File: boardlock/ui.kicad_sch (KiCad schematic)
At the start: 5 parts

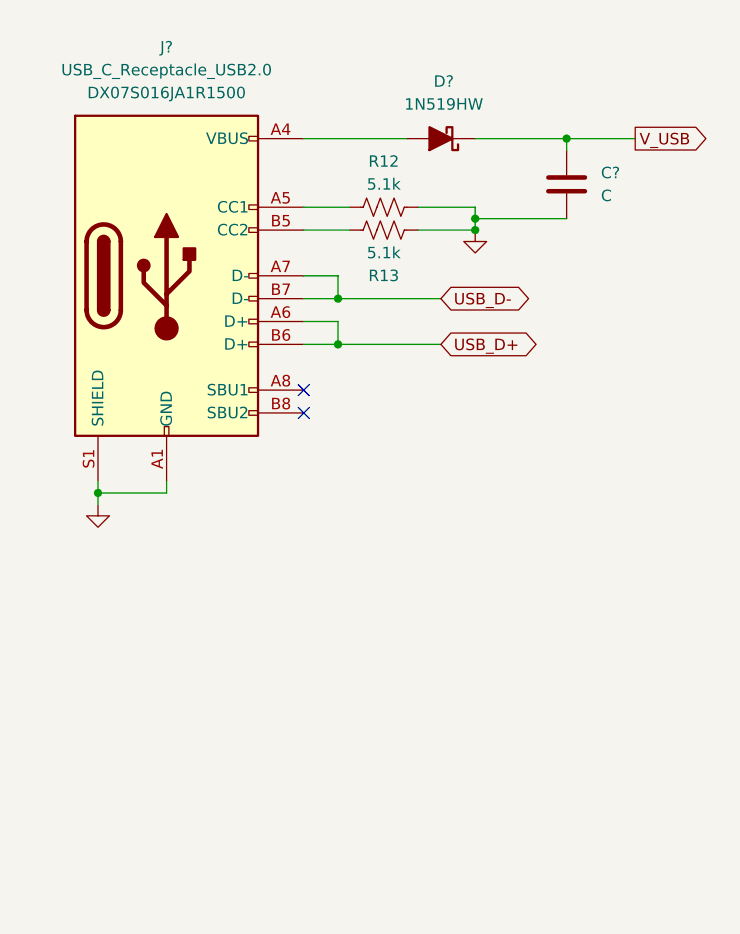
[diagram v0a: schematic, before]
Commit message: more Zecong edits
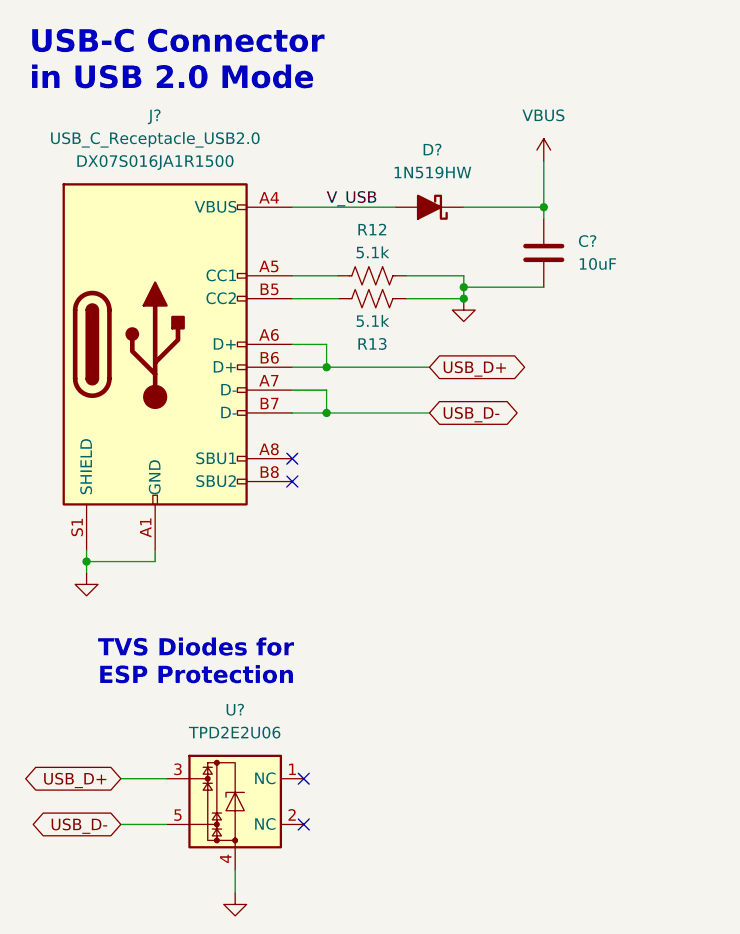
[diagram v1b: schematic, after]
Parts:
- removed C?: C, symbol Device:C
- added C?: 10uF, symbol Device:C
- added U?: TPD2E2U06, Package_TO_SOT_SMD:SOT-543, symbol Power_Protection:TPD2E2U06
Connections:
- net GND: now also C?.2, U?.4
- net USB_D+: now also U?.3
- net USB_D-: now also U?.5
- net V_USB: now also D?.2 (A), J?.A4 (VBUS), J?.A9 (VBUS), J?.B4 (VBUS), J?.B9 (VBUS); no longer D?.1 (K)
- new net VBUS: C?.1, D?.1 (K)
- no-connect marks 2 -> 4
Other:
- note added: "TVS Diodes for ESP Protection"
- note added: "USB-C Connector in USB 2.0 Mode"
- moved on the sheet: D?, J?, R12, R13

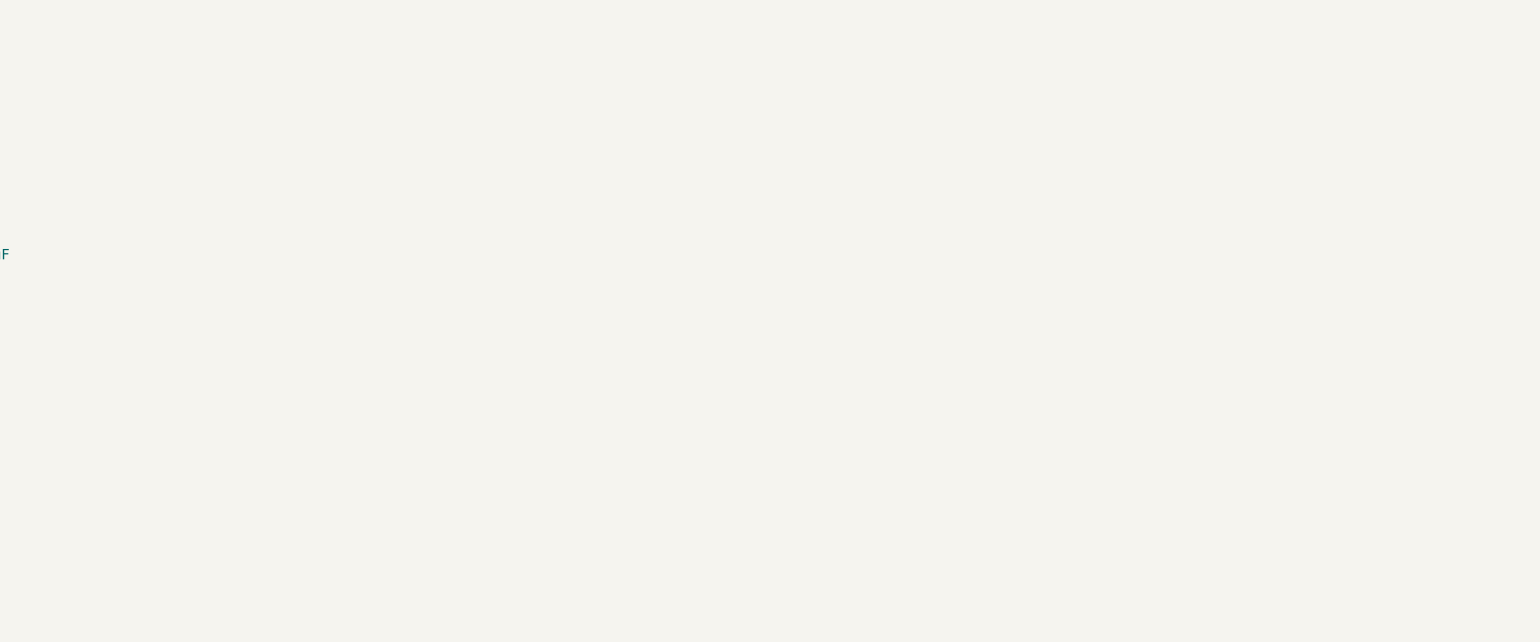
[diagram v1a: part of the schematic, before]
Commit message: buttons and stuff
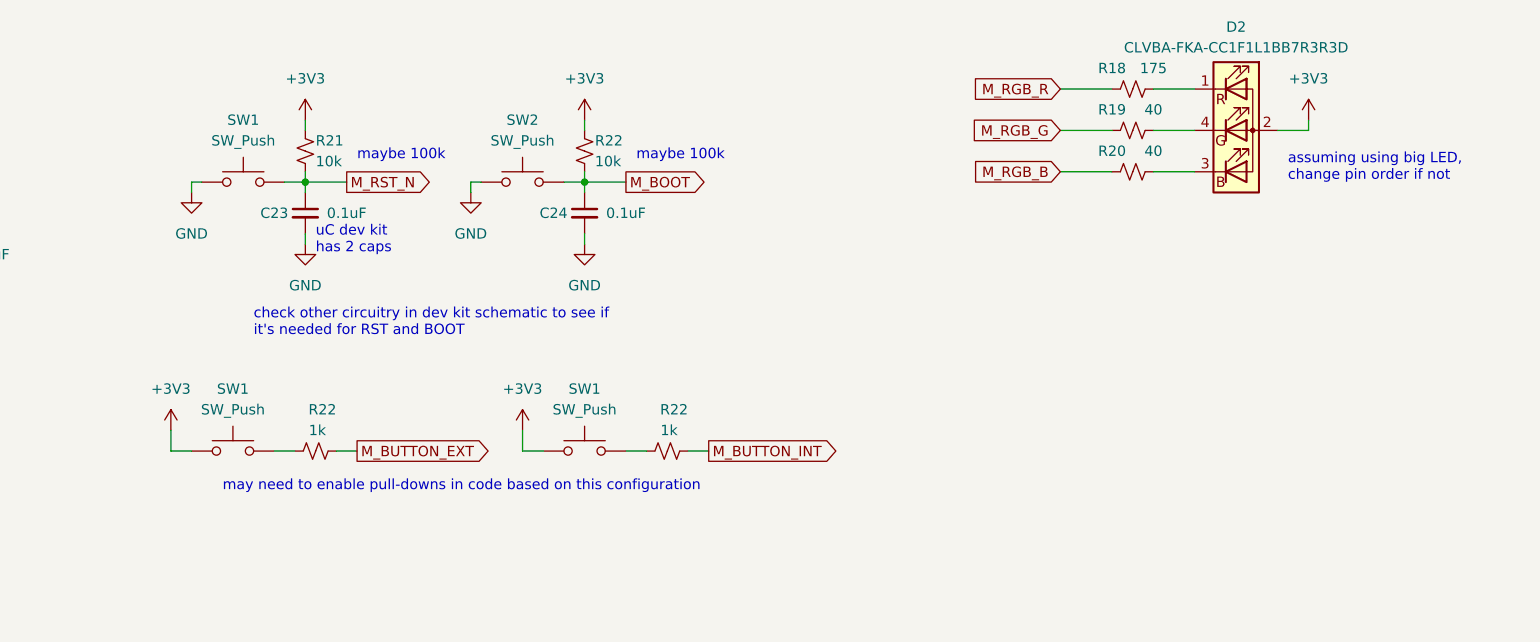
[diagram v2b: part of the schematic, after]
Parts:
- added C23, C24: 0.1uF, symbol Device:C_Small
- added D2: CLVBA-FKA-CC1F1L1BB7R3R3D, symbol Device:LED_RABG
- added R18: 175, symbol Device:R_Small_US
- added R19, R20: 40, symbol Device:R_Small_US
- added R21, R22: 10k, symbol Device:R_Small_US
- added R22 (x2): 1k, symbol Device:R_Small_US
- added SW1 (x3), SW2: SW_Push, symbol Switch:SW_Push
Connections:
- net GND: now also C23.2, C24.2, SW1.1, SW2.1
- new net: D2.1 (RK), R18.1
- new net: D2.3 (BK), R20.1
- new net: D2.4 (GK), R19.1
- new net: R22.1, SW1.2 (x2)
- new net +3V3: D2.2 (A), R21.1, R22.1, SW1.1, SW1.1
- new net M_BOOT: C24.1, R22.2, SW2.2
- new net M_BUTTON_EXT: R22.2
- new net M_BUTTON_INT: R22.2
- new net M_RGB_B: R20.2
- new net M_RGB_G: R19.2
- new net M_RGB_R: R18.2
- new net M_RST_N: C23.1, R21.2, SW1.2
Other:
- note added: "assuming using big LED, change pin order if not"
- note added: "check other circuitry in dev kit schematic to see if it's needed for RST and BOOT"
- note added: "may need to enable pull-downs in code based on this configuration"
- note added: "maybe 100k"
- note added: "uC dev kit has 2 caps"

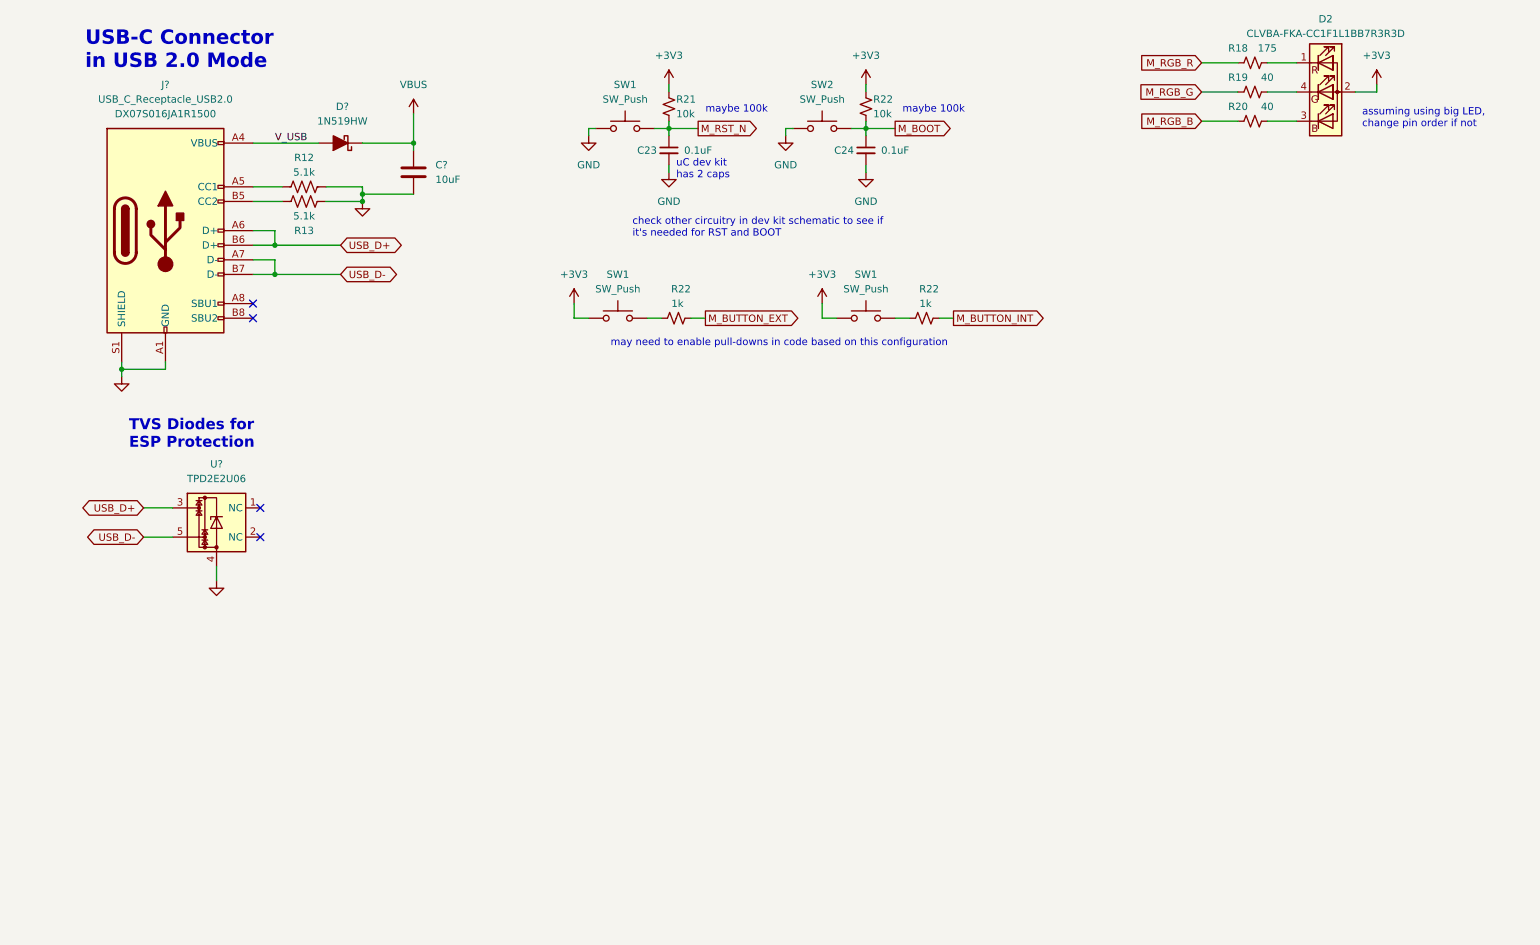
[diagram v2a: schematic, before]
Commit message: lab updates
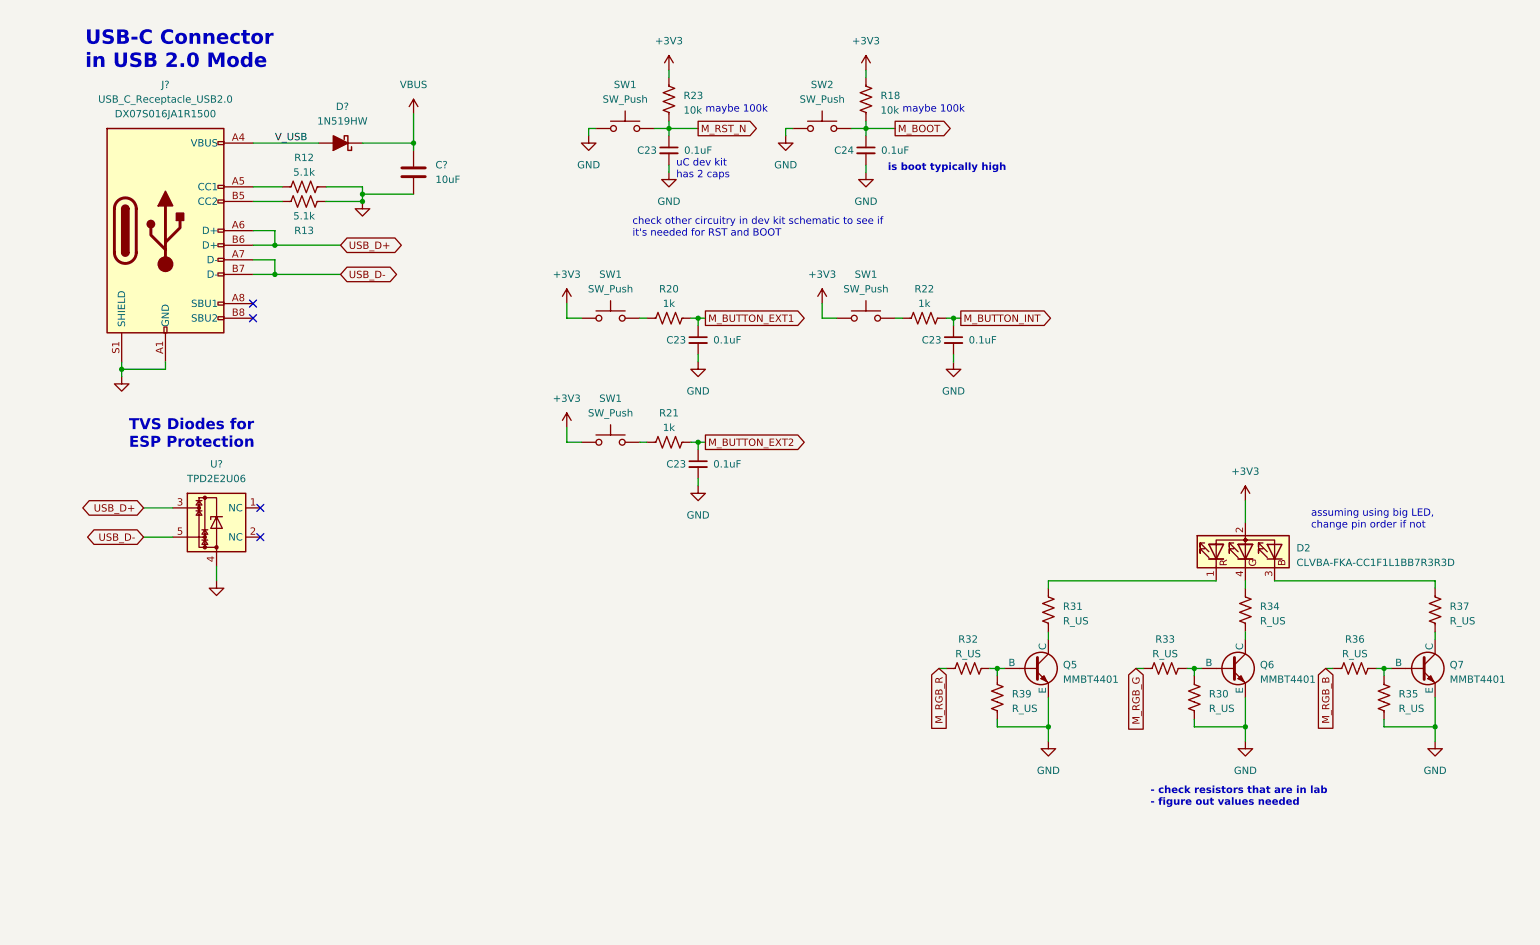
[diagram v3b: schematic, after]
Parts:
- removed R18: 175, symbol Device:R_Small_US
- removed R19, R20: 40, symbol Device:R_Small_US
- removed R21, R22: 10k, symbol Device:R_Small_US
- removed R22 (x2): 1k, symbol Device:R_Small_US
- removed SW1: SW_Push, symbol Switch:SW_Push
- added C23 (x3): 0.1uF, symbol Device:C_Small
- added Q5, Q6, Q7: MMBT4401, symbol Simulation_SPICE:NPN
- added R18, R23: 10k, symbol Device:R_US
- added R20, R21, R22: 1k, symbol Device:R_US
- added R30, R31, R32, R33, R34, R35, R36, R37, R39: R_US, symbol Device:R_US
- added SW1 (x2): SW_Push, symbol Switch:SW_Push
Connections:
- net +3V3: now also R18.1, R23.1, SW1.1, SW1.1
- net GND: now also C23.2, C23.2, C23.2, Q5.3 (E), Q6.3 (E), Q7.3 (E), R30.2, R35.2, R39.2
- net M_BOOT: now also R18.2
- net M_BUTTON_INT: now also C23.1, R22.2
- net M_RGB_B: now also R36.1
- net M_RGB_G: now also R33.1
- net M_RGB_R: now also R32.1
- net M_RST_N: now also R23.2
- net at D2.1 (RK): now also R31.1
- net at D2.3 (BK): now also R37.1
- net at D2.4 (GK): now also R34.1
- net at SW1.2: now also R20.1
- new net: Q6.1 (C), R34.2
- new net: Q6.2 (B), R30.1, R33.2
- new net: R21.1, SW1.2
- new net: Q5.1 (C), R31.2
- new net: Q5.2 (B), R32.2, R39.1
- new net: R22.1, SW1.2
- new net: Q7.1 (C), R37.2
- new net: Q7.2 (B), R35.1, R36.2
- new net M_BUTTON_EXT1: C23.1, R20.2
- new net M_BUTTON_EXT2: C23.1, R21.2
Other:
- note added: "- check resistors that are in lab - figure out values needed"
- note added: "is boot typically high"
- note removed: "may need to enable pull-downs in code based on this configuration"
- moved on the sheet: SW1

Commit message: not sure what I changed
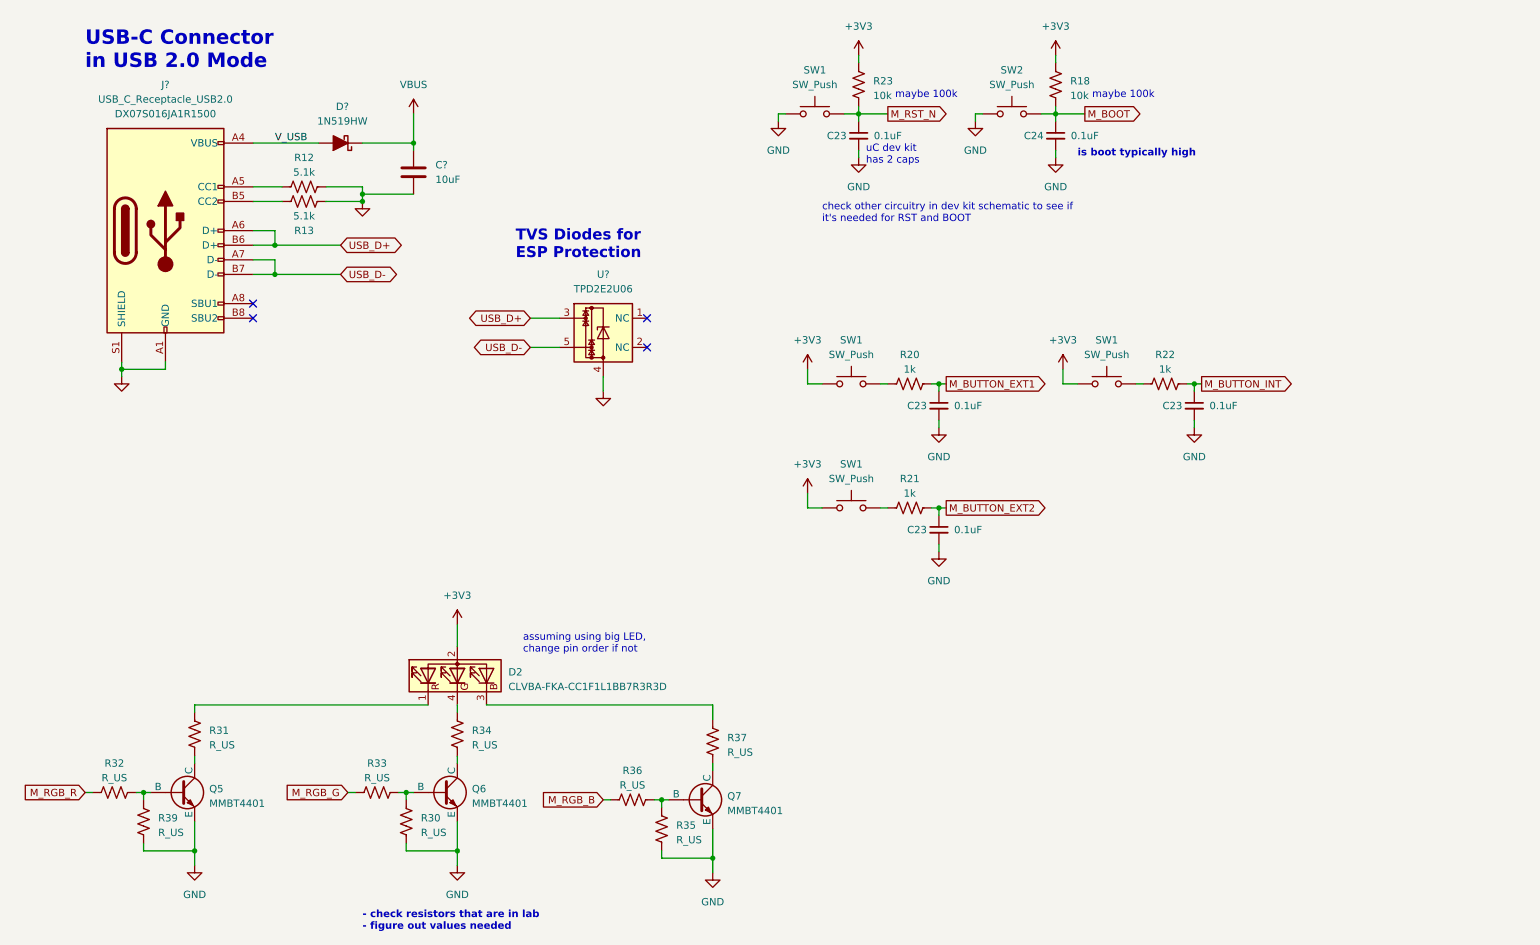
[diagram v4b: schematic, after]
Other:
- moved on the sheet: C23, C24, D2, Q5, Q6, Q7, R18, R20, R21, R22, R23, R30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
